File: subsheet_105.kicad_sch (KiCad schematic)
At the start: 16 parts, among them T01 BC547B, T02 BC547B, T03 BC547B

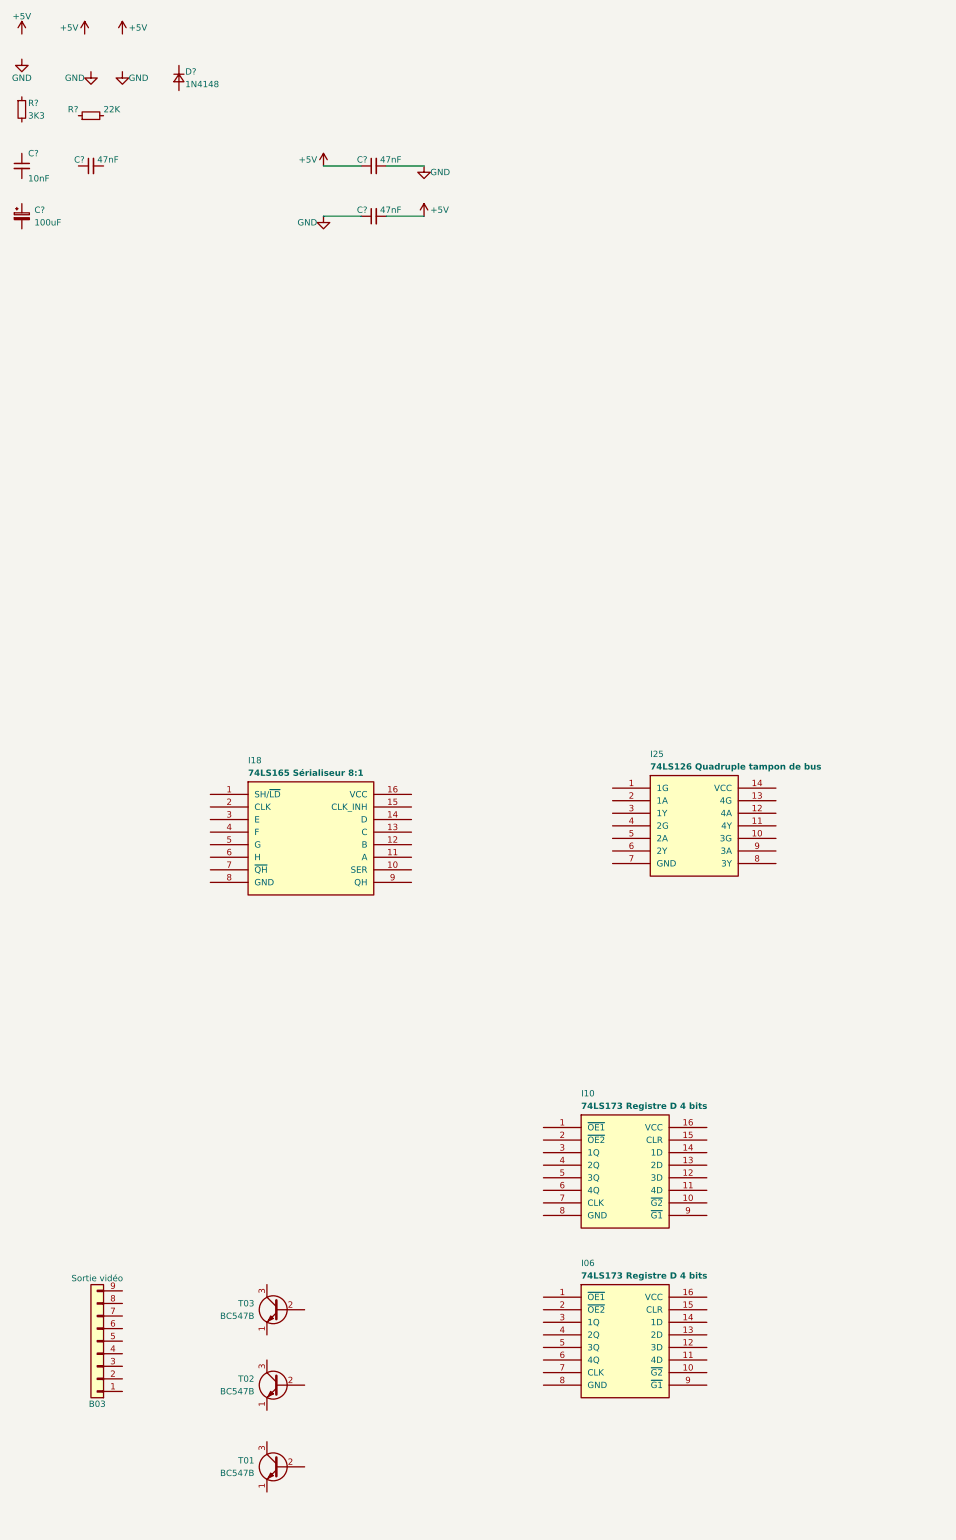
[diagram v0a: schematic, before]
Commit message: continue circuit vidéo
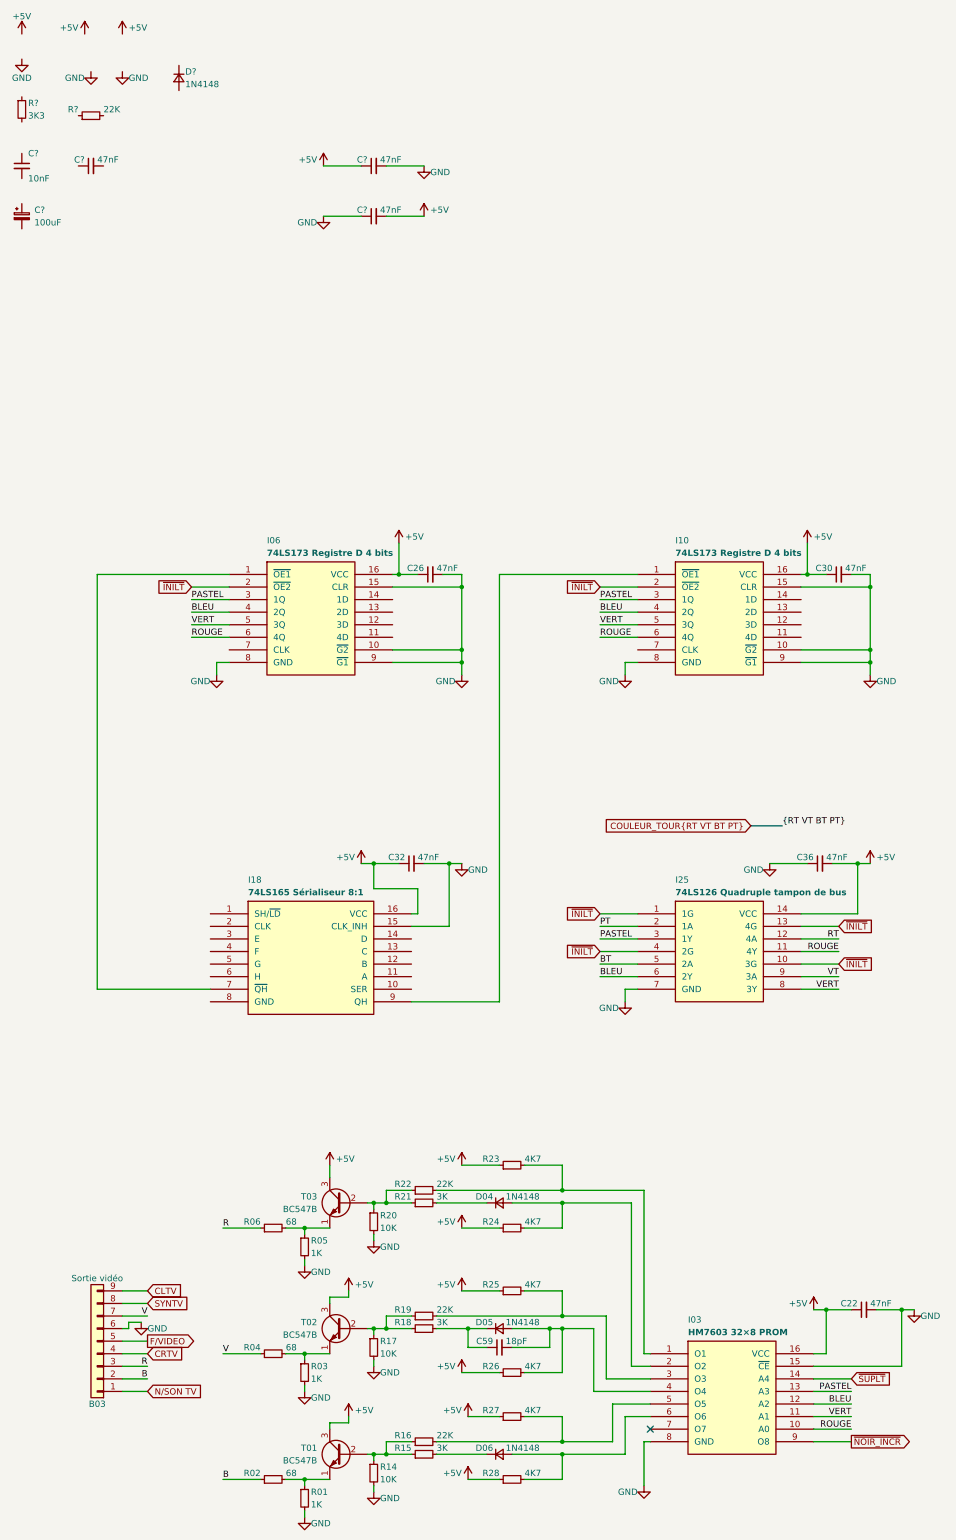
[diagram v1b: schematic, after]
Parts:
- added C22, C26, C30, C32, C36: 47nF, symbol Device:C_Small
- added C59: 18pF, symbol Device:C_Small
- added D04, D05, D06: 1N4148, symbol Device:D_Small
- added I03: HM7603 32×8 PROM, Package_DIP:DIP-16_W7.62mm_LongPads, symbol hm7603:HM7603_32×8_PROM_THREE-STATE_OUTPUTS_PHY
- added R01, R03, R05: 1K, symbol Device:R_Small
- added R02, R04, R06: 68, symbol Device:R_Small
- added R14, R17, R20: 10K, symbol Device:R_Small
- added R15, R18, R21: 3K, symbol Device:R_Small
- added R16, R19, R22: 22K, symbol Device:R_Small
- added R23, R24, R25, R26, R27, R28: 4K7, symbol Device:R_Small
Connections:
- net +5V: now also I06.16 (VCC), I10.16 (VCC), I18.16 (VCC), I25.14 (VCC), T01.3 (C), T02.3 (C), T03.3 (C), C22.1, C26.1, C30.1, C32.1, C36.2, I03.16 (VCC), R23.1, R24.1, R25.1, R26.1, R27.1, R28.1
- net GND: now also B03.6 (Pin_6), I06.10 (~{G2}), I06.15 (CLR), I06.8 (GND), I06.9 (~{G1}), I10.10 (~{G2}), I10.15 (CLR), I10.8 (GND), I10.9 (~{G1}), I18.15 (CLK_INH), I25.7 (GND), C22.2, C26.2, C30.2, C32.2, C36.1, I03.15 (~{CE}), I03.8 (GND), R01.2, R03.2, R05.2, R14.2, R17.2, R20.2
- net at T01.1 (E): now also R01.1, R02.2
- net at T01.2 (B): now also R14.1, R15.1, R16.1
- net ~{INILT}: now reaches I25.1 (1G)
- net ~{INILT}: now also I06.2 (~{OE2}), I10.2 (~{OE2}), I25.10 (3G), I25.13 (4G), I25.4 (2G)
- net ROUGE: now reaches I25.11 (4Y)
- net ROUGE: now also I06.6 (4Q), I10.6 (4Q), I03.10 (A0)
- net RT: now reaches I25.12 (4A)
- net PT: now reaches I25.2 (1A)
- net PASTEL: now reaches I25.3 (1Y)
- net PASTEL: now also I06.3 (1Q), I10.3 (1Q), I03.13 (A3)
- net BT: now reaches I25.5 (2A)
- net BLEU: now reaches I25.6 (2Y)
- net BLEU: now also I06.4 (2Q), I10.4 (2Q), I03.12 (A2)
- net VERT: now reaches I25.8 (3Y)
- net VERT: now also I06.5 (3Q), I10.5 (3Q), I03.11 (A1)
- net VT: now reaches I25.9 (3A)
- net at I06.1 (~{OE1}): now also I18.7 (~{QH})
- net at T03.1 (E): now also R05.1, R06.2
- net at T03.2 (B): now also R20.1, R21.1, R22.1
- net at I18.9 (QH): now also I10.1 (~{OE1})
- net at T02.1 (E): now also R03.1, R04.2
- net at T02.2 (B): now also R17.1, R18.1, R19.1
- net N/SON TV: now reaches B03.1 (Pin_1)
- net B: now reaches B03.2 (Pin_2)
- net B: now also R02.1
- net R: now reaches B03.3 (Pin_3)
- net R: now also R06.1
- net CRTV: now reaches B03.4 (Pin_4)
- net F/VIDEO: now reaches B03.5 (Pin_5)
- net V: now reaches B03.7 (Pin_7)
- net V: now also R04.1
- net SYNTV: now reaches B03.8 (Pin_8)
- net CLTV: now reaches B03.9 (Pin_9)
- new net: I03.1 (O1), R22.2, R23.2
- new net: D04.2 (A), I03.2 (O2), R24.2
- new net: I03.3 (O3), R19.2, R25.2
- new net: C59.2, D05.2 (A), I03.4 (O4), R26.2
- new net: I03.5 (O5), R16.2, R27.2
- new net: D06.2 (A), I03.6 (O6), R28.2
- new net: C59.1, D05.1 (K), R18.2
- new net: D04.1 (K), R21.2
- new net: D06.1 (K), R15.2
- new net ~{NOIR_INCR}: I03.9 (O8)
- new net ~{SUPLT}: I03.14 (A4)
- no-connect marks 0 -> 1
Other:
- moved on the sheet: I06, I10, I18, I25, T01, T02, T03
